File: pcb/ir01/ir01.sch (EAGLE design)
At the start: 9 parts

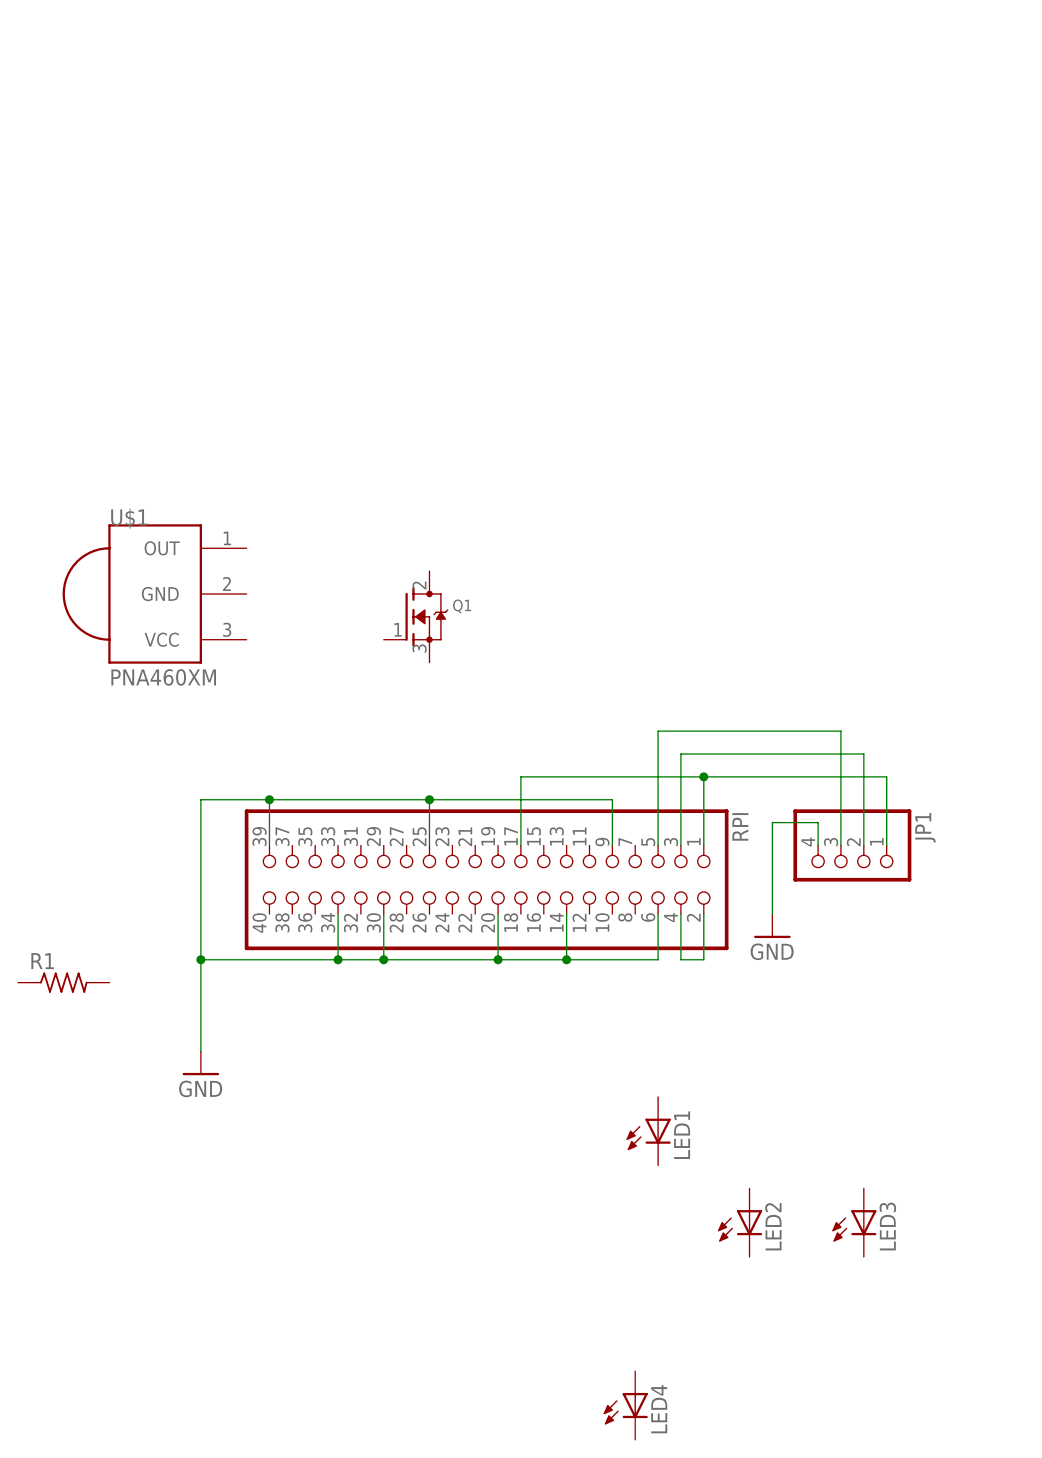
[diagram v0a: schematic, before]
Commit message: pcb
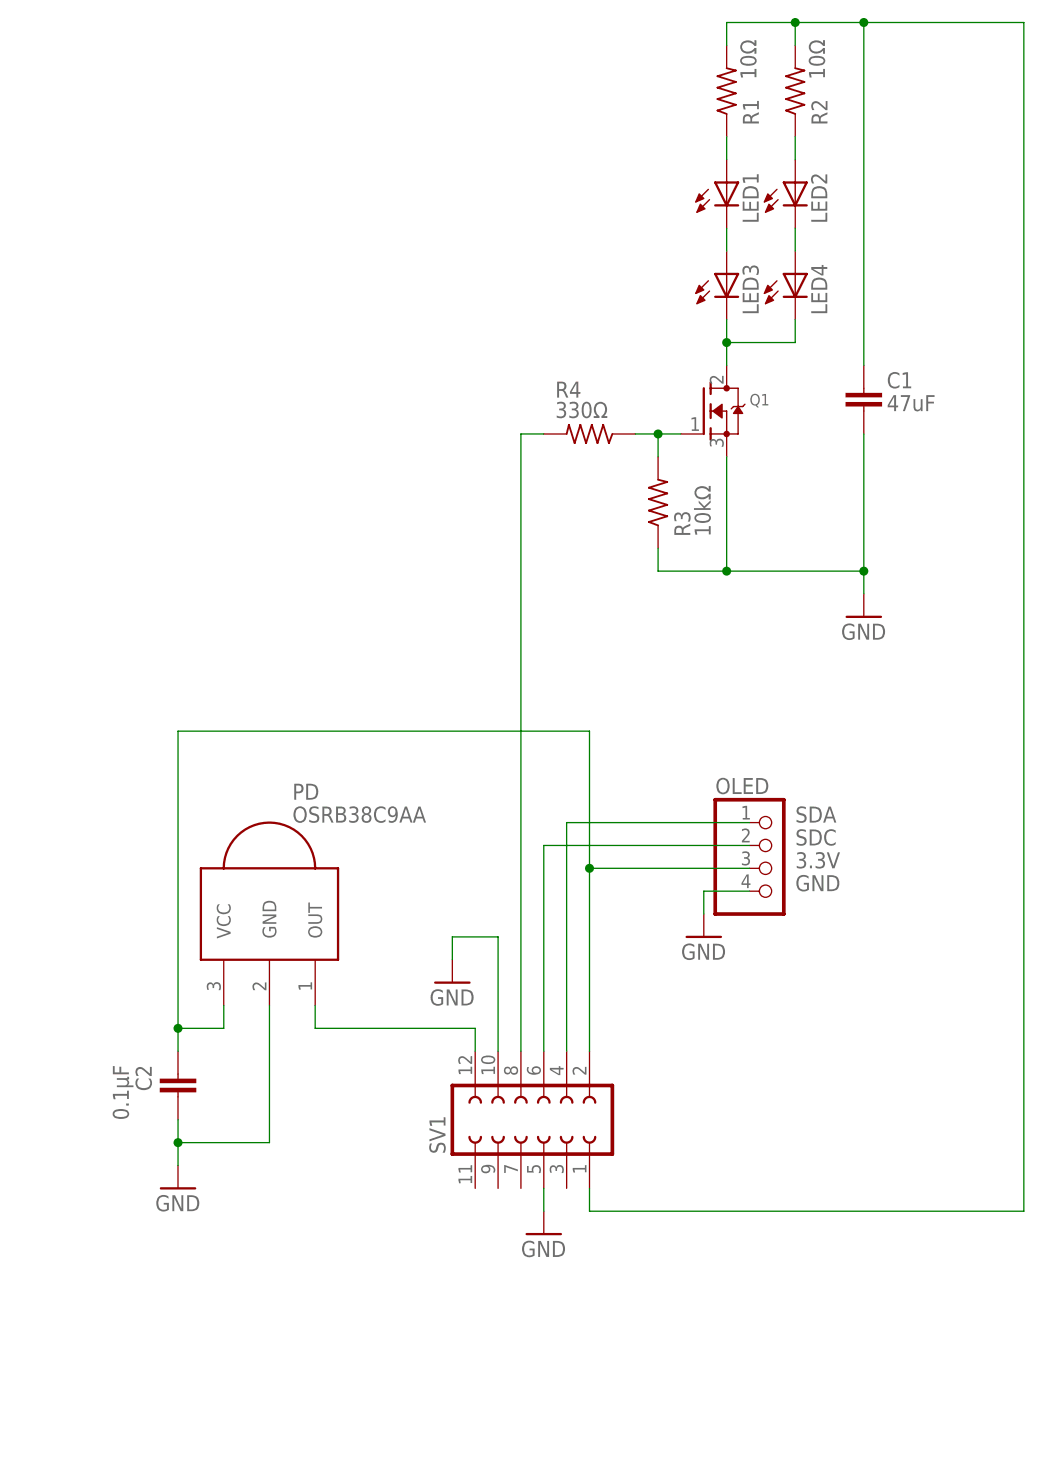
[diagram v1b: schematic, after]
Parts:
- removed JP1: (no value), pinhead:PINHD-1X4
- removed RPI: (no value), adafruit:PINHD-2X20-BIG
- removed U$1: PNA460XM, adafruit:PNA460XM
- added C1: 47uF, rcl:C-EU025-025X050
- added C2: 0.1μF, rcl:C-EU025-025X050
- added OLED: (no value), pinhead:PINHD-1X4
- added PD: OSRB38C9AA, adafruit:PNA460XM
- added R2: 10Ω, rcl:R-US_0204/5
- added R3: 10kΩ, rcl:R-US_0204/5
- added R4: 330Ω, rcl:R-US_0204/5
- added SV1: (no value), con-lsta:FE06-2
- R1: value (none) -> 10Ω
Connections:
- removed net N$6: RPI.2, RPI.4
- new net 3.3V: C2.1, OLED.3, PD.VCC, SV1.2
- new net 5V: C1.1, R1.2, R2.2, SV1.1
- new net N$4: LED1.A, R1.1
- new net N$5: LED2.A, R2.1
- new net N$7: LED1.C, LED3.A
- new net N$8: LED2.C, LED4.A
- new net N$9: LED3.C, LED4.C, Q1.D
- new net SDA: OLED.1, SV1.4
- new net SDC: OLED.2, SV1.6
- net GND: now also C1.2, C2.2, OLED.4, PD.GND, Q1.S, R3.1, SV1.10, SV1.5; no longer JP1.4, RPI.14, RPI.20, RPI.25, RPI.30, RPI.34, RPI.39, RPI.6, RPI.9
- net N$1: now also Q1.G, R3.2, R4.1; no longer JP1.1, RPI.1, RPI.17
- net N$2: now also PD.OUT, SV1.12; no longer JP1.2, RPI.3
- net N$3: now also R4.2, SV1.8; no longer JP1.3, RPI.5
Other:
- moved on the sheet: LED1, LED2, LED3, LED4, Q1, R1
